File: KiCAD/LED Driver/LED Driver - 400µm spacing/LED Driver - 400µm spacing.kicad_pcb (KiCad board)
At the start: 2 copper layers, 16.5 x 9 mm, 16 parts, among them Q1 Q_NMOS_GSD, U1 LP5868TRKPR, U2 ATtiny3226, U3 XC61GC3002HR-G

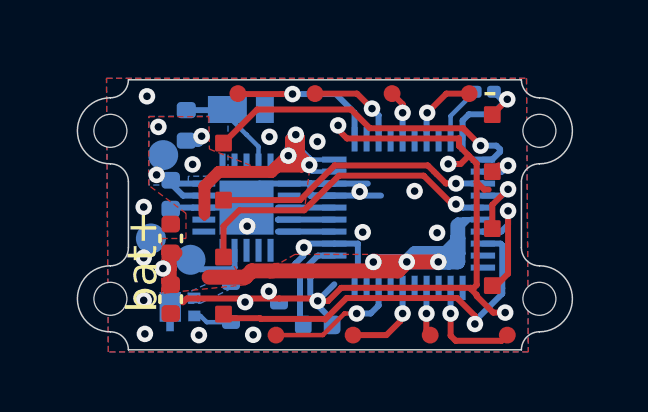
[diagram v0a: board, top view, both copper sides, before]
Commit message: Working draft of programmer/charger board
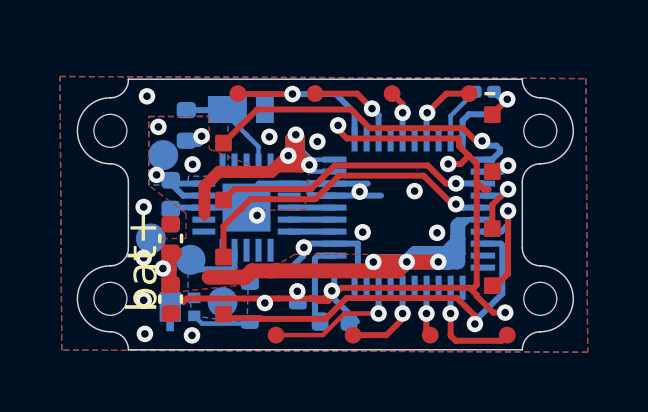
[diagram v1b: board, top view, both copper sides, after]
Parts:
- added BT1: LiPo Cell, Custom:LPM0940, B.Cu at (54.7, 34.2)
- TP2: footprint Custom:1mm pad -> Custom:1mm pad x4
- moved Q1 0.63 mm to (51.0, 37.1)
- moved C2 0.57 mm to (53.0, 37.8)
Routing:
- net Net-(Q1-G): track 1.31 -> 2.05 mm
- net GND: track 41.5 -> 41.2 mm, vias 21 -> 20
